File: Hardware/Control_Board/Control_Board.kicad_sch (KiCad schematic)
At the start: 1 part, among them IC2 ARD-NANO30NP

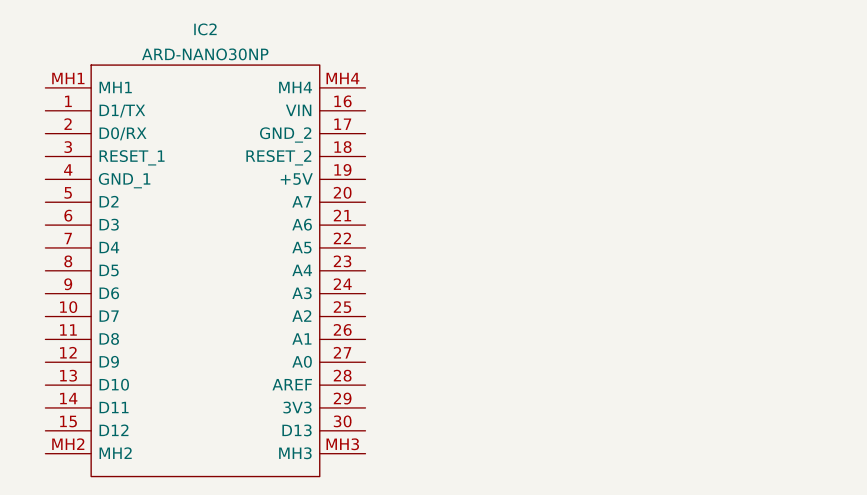
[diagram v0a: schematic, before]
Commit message: Control board updates
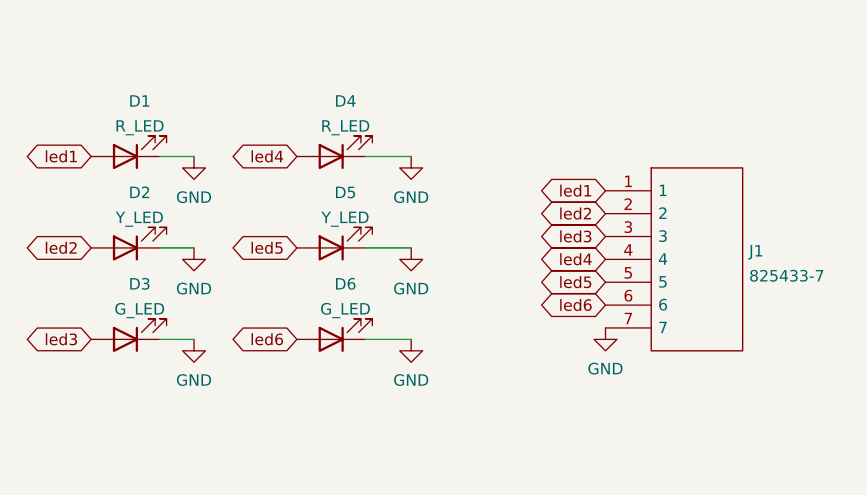
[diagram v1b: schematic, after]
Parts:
- removed IC2: ARD-NANO30NP, ARDNANO30NP, symbol Samacsys:ARD-NANO30NP
- added D1, D4: R_LED, symbol Device:LED
- added D2, D5: Y_LED, symbol Device:LED
- added D3, D6: G_LED, symbol Device:LED
- added J1: 825433-7, 8254337, symbol Samacsys:825433-7
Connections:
- new net GND: D1.1 (K), D2.1 (K), D3.1 (K), D4.1 (K), D5.1 (K), D6.1 (K), J1.7
- new net led1: D1.2 (A), J1.1
- new net led2: D2.2 (A), J1.2
- new net led3: D3.2 (A), J1.3
- new net led4: D4.2 (A), J1.4
- new net led5: D5.2 (A), J1.5
- new net led6: D6.2 (A), J1.6

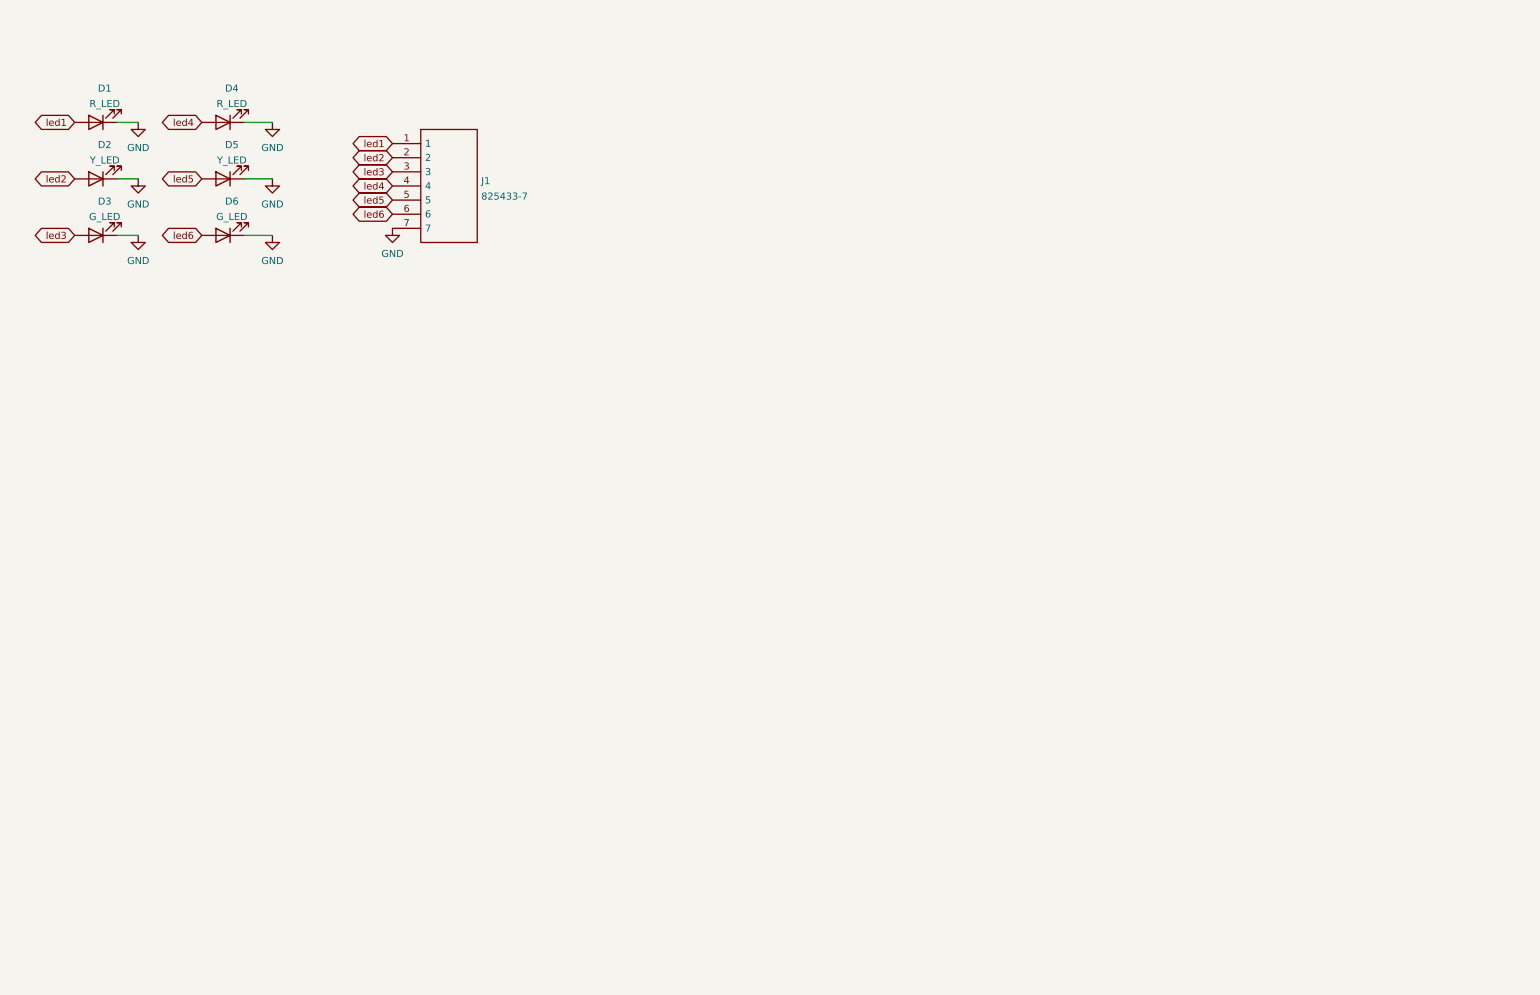
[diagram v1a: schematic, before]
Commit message: Sch rev 1 ready for review
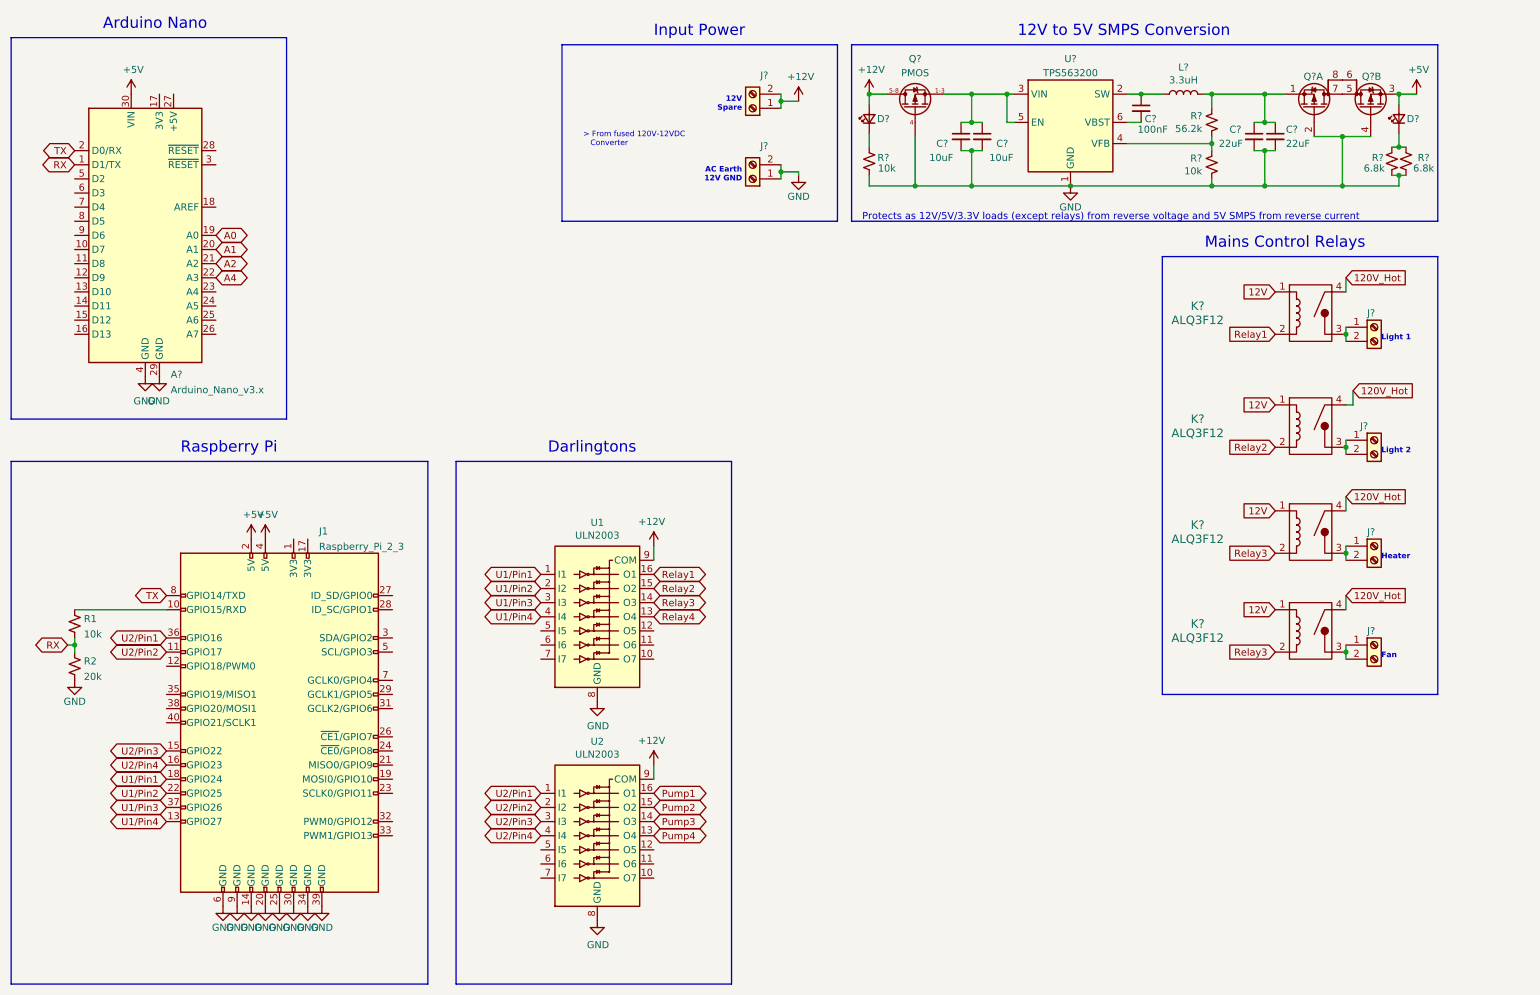
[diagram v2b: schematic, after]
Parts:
- removed D1, D4: R_LED, symbol Device:LED
- removed D2, D5: Y_LED, symbol Device:LED
- removed D3, D6: G_LED, symbol Device:LED
- removed J1: 825433-7, 8254337, symbol Samacsys:825433-7
- added A?: Arduino_Nano_v3.x, Module:Arduino_Nano, symbol MCU_Module:Arduino_Nano_v3.x
- added C? (x2): 22uF, Capacitor_SMD:C_1206_3216Metric, symbol OzoneController-rescue:C_Small-Device-OzoneController-rescue
- added C?: 100nF, Capacitor_SMD:C_0603_1608Metric, symbol OzoneController-rescue:C_Small-Device-OzoneController-rescue
- added C? (x2): 10uF, Capacitor_SMD:C_1206_3216Metric, symbol OzoneController-rescue:C_Small-Device-OzoneController-rescue
- added D? (x2): LED_Red_power, LED_SMD:LED_0603_1608Metric, symbol Device:LED_Small
- added J1: Raspberry_Pi_2_3, symbol Connector:Raspberry_Pi_2_3
- added J? (x4): Term_01x02, 1792863-2term_power:1792863, symbol Connector:Screw_Terminal_01x02
- added J? (x2): Screw_Terminal_01x02, TBL004-508-02BE-2GY:CUI_TBL004-508-02BE-2GY, symbol Connector:Screw_Terminal_01x02
- added K? (x4): ALQ3F12, ALQ3F12:ALQ3F12, symbol OzoneController-rescue:ALQ3F12-ALQ3F12-OzoneController-rescue
- added L?: 3.3uH, Inductor_SMD:L_10.4x10.4_H4.8, symbol OzoneController-rescue:L-Device-OzoneController-rescue
- added Q? (x2): Q_Dual_PMOS_S1G1S2G2D2D2D1D1, Package_SO:SOP-8_3.9x4.9mm_P1.27mm, symbol Device:Q_Dual_PMOS_S1G1S2G2D2D2D1D1
- added Q?: PMOS, Package_SO:SOIC-8_3.9x4.9mm_P1.27mm, symbol Project_Library:PMOS_AO4407A
- added R1: 10k, symbol Device:R_Small_US
- added R2: 20k, symbol Device:R_Small_US
- added R? (x2): 6.8k, Resistor_SMD:R_0402_1005Metric, symbol Device:R_Small_US
- added R?: 56.2k, Resistor_SMD:R_0402_1005Metric, symbol Device:R_Small_US
- added R? (x2): 10k, Resistor_SMD:R_0402_1005Metric, symbol Device:R_Small_US
- added U1, U2: ULN2003, Package_SO:SOIC-16_3.9x9.9mm_P1.27mm, symbol OzoneController-rescue:ULN2003-Transistor_Array-OzoneController-rescue
- added U?: TPS563200, Package_TO_SOT_SMD:SOT-23-6, symbol Regulator_Switching:TPS563200
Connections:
- net GND: now also A?.29 (GND), A?.4 (GND), C?.2, C?.2, C?.2, C?.2, J1.14 (GND), J1.20 (GND), J1.25 (GND), J1.30 (GND), J1.34 (GND), J1.39 (GND), J1.6 (GND), J1.9 (GND), J?.1 (Pin_1), J?.2 (Pin_2), Q?.2 (G), Q?.4, Q?.4 (G), R2.2, R?.1, R?.1, R?.1, R?.1, U1.8 (GND), U2.8 (GND), U?.1 (GND)
- new net: C?.1, L?.1, U?.2 (SW)
- new net: C?.1, C?.1, Q?.1 (D), Q?.2 (G), Q?.3 (eS), U?.3 (VIN), U?.5 (EN)
- new net: R?.1, R?.2, U?.4 (VFB)
- new net: C?.2, U?.6 (VBST)
- new net: J?.1 (Pin_1), J?.2 (Pin_2), K?.3 (NO) (x4)
- new net: D?.1 (K), R?.2, R?.2
- new net: C?.1, C?.1, L?.2, Q?.1 (S), R?.2
- new net: Q?.5 (D), Q?.7 (D)
- new net: Q?.6 (G), Q?.8 (G)
- new net: J1.10 (GPIO15/RXD), R1.1
- new net: D?.1 (K), R?.2
- new net +12V: D?.2 (A), J?.1 (Pin_1), J?.2 (Pin_2), Q?.5, Q?.6, Q?.7, Q?.8, U1.9 (COM), U2.9 (COM)
- new net +5V: A?.30 (VIN), D?.2 (A), J1.2 (5V), J1.4 (5V), Q?.3 (S)
- new net 120V_Hot: K?.4 (COM), K?.4 (COM), K?.4 (COM), K?.4 (COM)
- new net 12V: K?.1 (Coil), K?.1 (Coil), K?.1 (Coil), K?.1 (Coil)
- new net A0: A?.19 (A0)
- new net A1: A?.20 (A1)
- new net A2: A?.21 (A2)
- new net A4: A?.22 (A3)
- new net Pump1: U2.16 (O1)
- new net Pump2: U2.15 (O2)
- new net Pump3: U2.14 (O3)
- new net Pump4: U2.13 (O4)
- new net RX: A?.1 (D1/TX), R1.2, R2.1
- new net Relay1: K?.2 (Coil), U1.16 (O1)
- new net Relay2: K?.2 (Coil), U1.15 (O2)
- new net Relay3: K?.2 (Coil), K?.2 (Coil), U1.14 (O3)
- new net Relay4: U1.13 (O4)
- new net TX: A?.2 (D0/RX), J1.8 (GPIO14/TXD)
- new net U1/Pin1: J1.18 (GPIO24), U1.1 (I1)
- new net U1/Pin2: J1.22 (GPIO25), U1.2 (I2)
- new net U1/Pin3: J1.37 (GPIO26), U1.3 (I3)
- new net U1/Pin4: J1.13 (GPIO27), U1.4 (I4)
- new net U2/Pin1: J1.36 (GPIO16), U2.1 (I1)
- new net U2/Pin2: J1.11 (GPIO17), U2.2 (I2)
- new net U2/Pin3: J1.15 (GPIO22), U2.3 (I3)
- new net U2/Pin4: J1.16 (GPIO23), U2.4 (I4)
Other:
- note added: "12V Spare"
- note added: "12V to 5V SMPS Conversion"
- note added: "> From fused 120V-12VDC Converter"
- note added: "AC Earth 12V GND"
- note added: "Arduino Nano"
- note added: "Darlingtons"
- note added: "Fan"
- note added: "Heater"
- note added: "Input Power"
- note added: "Light 1"
- note added: "Light 2"
- note added: "Mains Control Relays"
- note added: "Protects as 12V/5V/3.3V loads (except relays) from reverse voltage and 5V SMPS from reverse current"
- note added: "Raspberry Pi"
